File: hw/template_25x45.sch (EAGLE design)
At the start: 23 parts, among them J1 GROVE-4P-2.0-3470130P1, J2 GROVE-4P-2.0-3470130P1

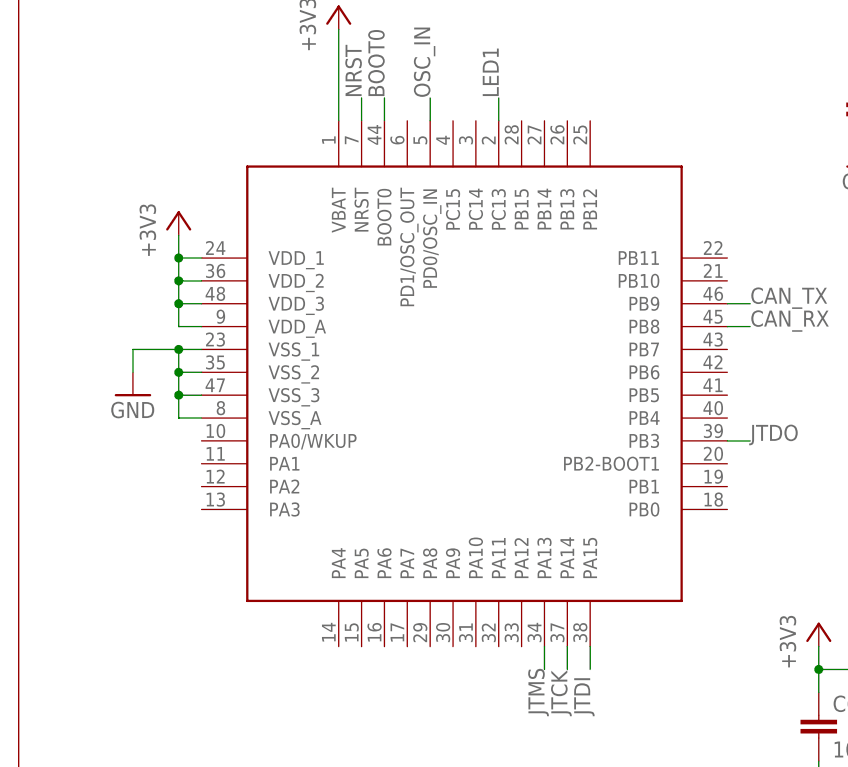
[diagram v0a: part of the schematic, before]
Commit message: updated to STM32F303 family
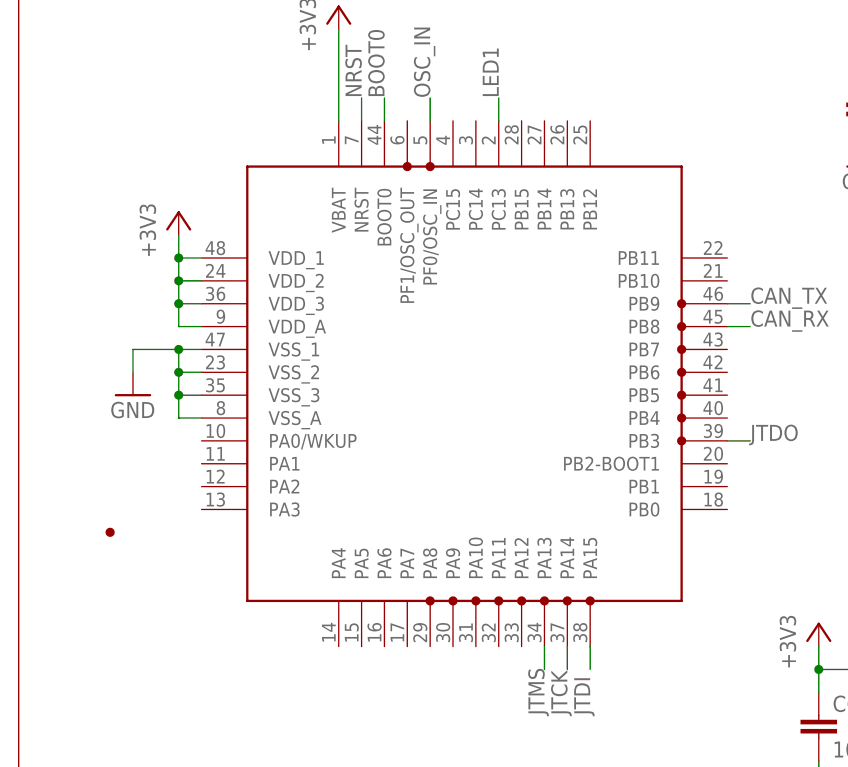
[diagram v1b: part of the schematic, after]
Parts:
- U$6: value STM32F103CX -> STM32F303C; device st:STM32F103CX -> st:STM32F303C
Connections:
- net OSC_IN: now also U$6.PF0/OSC_IN; no longer U$6.PD0/OSC_IN
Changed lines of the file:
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@@
 <part name="J1" library="OPL Eagle Library" deviceset="GROVE-4P-2.0" device="-3470130P1"/>
 <part name="+3V7" library="supply1" deviceset="+3V3" device=""/>
-<part name="U$6" library="st" deviceset="STM32F103CX" device=""/>
+<part name="U$6" library="st" deviceset="STM32F303C" device=""/>
 <part name="FRAME1" library="frames" deviceset="DINA3_L" device=""/>
 <part name="GND13" library="supply" deviceset="GND" device=""/>
@@
 <wire x1="50.8" y1="236.22" x2="50.8" y2="238.76" width="0.1524" layer="91"/>
 <label x="50.8" y="238.76" size="1.778" layer="95" rot="R90"/>
-<pinref part="U$6" gate="G$1" pin="PD0/OSC_IN"/>
-</segment>
-<segment>
+<pinref part="U$6" gate="G$1" pin="PF0/OSC_IN"/>
+</segment>
+<segment>
